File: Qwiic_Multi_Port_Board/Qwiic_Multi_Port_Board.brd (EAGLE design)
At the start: 25.4 x 25.4 mm, 10 parts, among them J1 QWIIC_RIGHT_ANGLE, J2 QWIIC_RIGHT_ANGLE, J3 QWIIC_RIGHT_ANGLE, J4 QWIIC_RIGHT_ANGLE

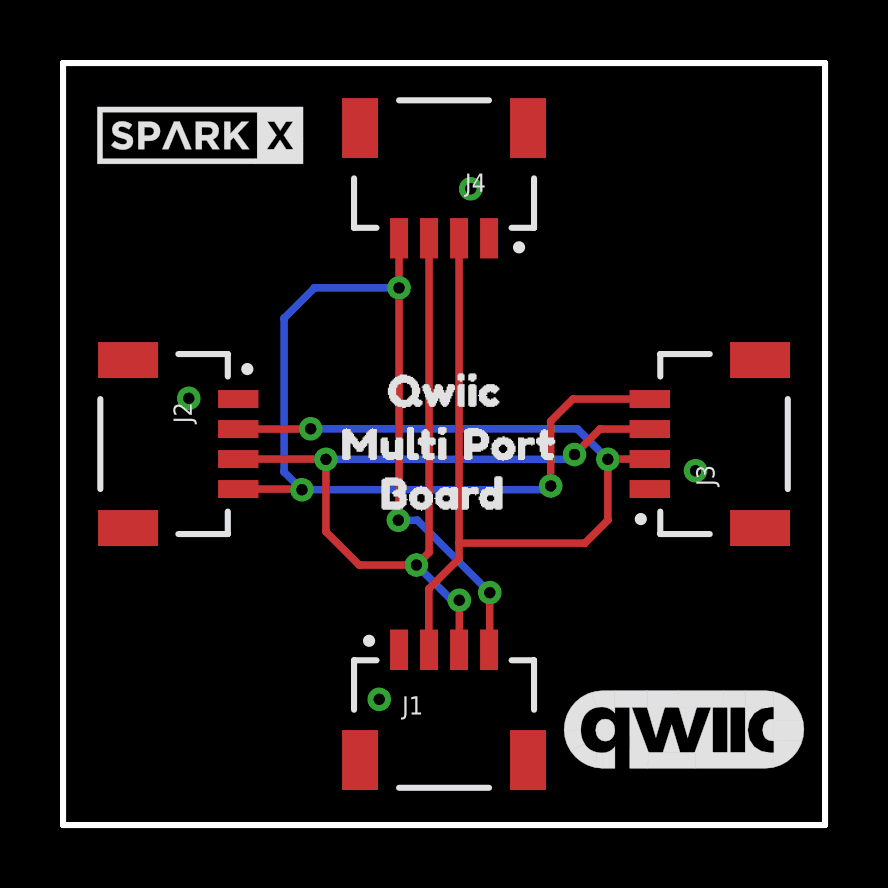
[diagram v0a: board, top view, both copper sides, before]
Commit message: Finishing touches
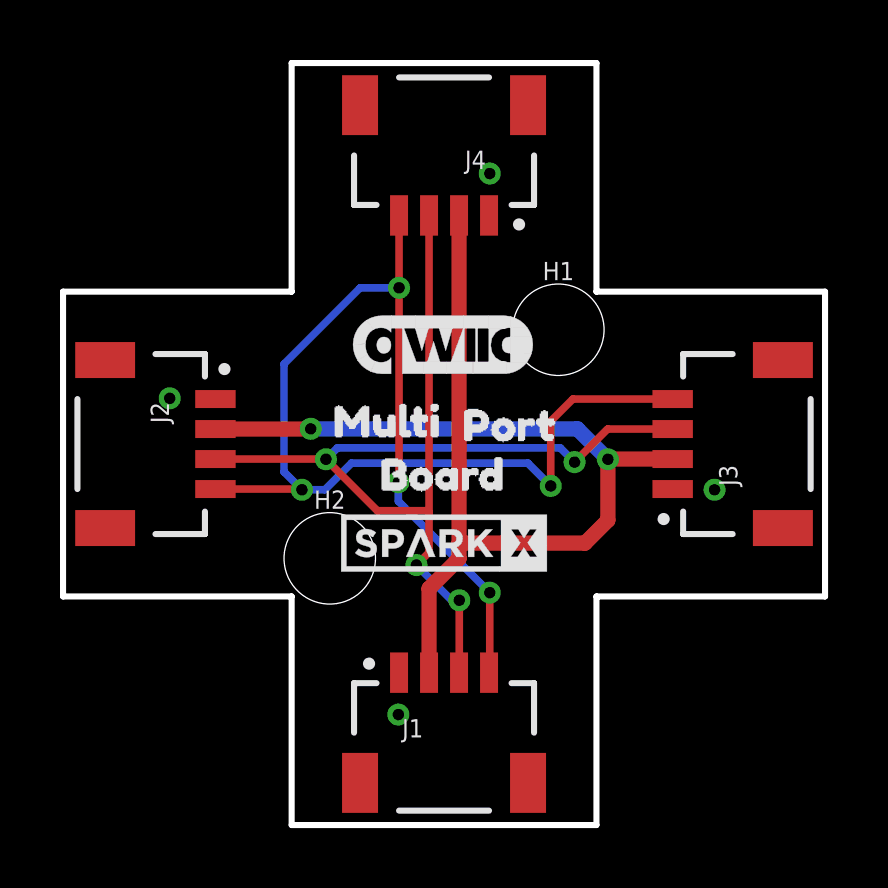
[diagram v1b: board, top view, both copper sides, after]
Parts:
- added H1, H2: STAND-OFFTIGHT, SparkFun-Hardware:STAND-OFF-TIGHT
- added U$10: (no value), SparkX:SPARKX-SMALL
- added U$7: (no value), buzzard_labels (75):MULTI1
- added U$8: (no value), buzzard_labels (75):PORT2
- added U$9: (no value), buzzard_labels (75):BOARD3
- U$1: device SparkFun-Aesthetics:QWIIC_8MM -> SparkFun-Aesthetics:QWIIC_6MM
- U$3: device buzzard_labels (75):QWIIC0 -> SparkFun-Aesthetics:QWIIC_6MM
- moved U$2 15.8 mm to (12.7, 9.40)
- moved U$1 15.1 mm to (12.7, 16.0)
- moved U$3 3.07 mm to (12.6, 16.0), flipped to the bottom
- moved U$4 0.80 mm to (8.13, 13.5)
- moved J3 0.76 mm to (20.3, 12.7)
- moved J4 0.76 mm to (12.7, 20.3)
- moved J1 0.76 mm to (12.7, 5.08)
- moved J2 0.76 mm to (5.08, 12.7)
- moved U$5 0.64 mm to (12.4, 13.3)
- moved U$6 0.63 mm to (9.65, 11.7)
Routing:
- net 3.3V: track 35.6 -> 38.6 mm
- net SCL: track 41.8 -> 44.2 mm
- net SDA: track 34.7 -> 36.4 mm
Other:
- outline, holes or cut-outs redrawn
